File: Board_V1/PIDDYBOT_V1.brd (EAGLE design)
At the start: 48 x 76 mm, 76 parts, among them IC1 FT232RLSSOP, IC2 LMV358, IC3 LM1117, Q1 MOSFET-PCHANNELSMD, Q2 MOSFET-NCHANNELSMD, Q3 MOSFET-NCHANNELSMD, U1 MPU-6050-1, U2 MIC5205, U3 ATMEGA328, U4 TB6621FNG, U5 BLUETOOTH-RN41, Y1 16MHz

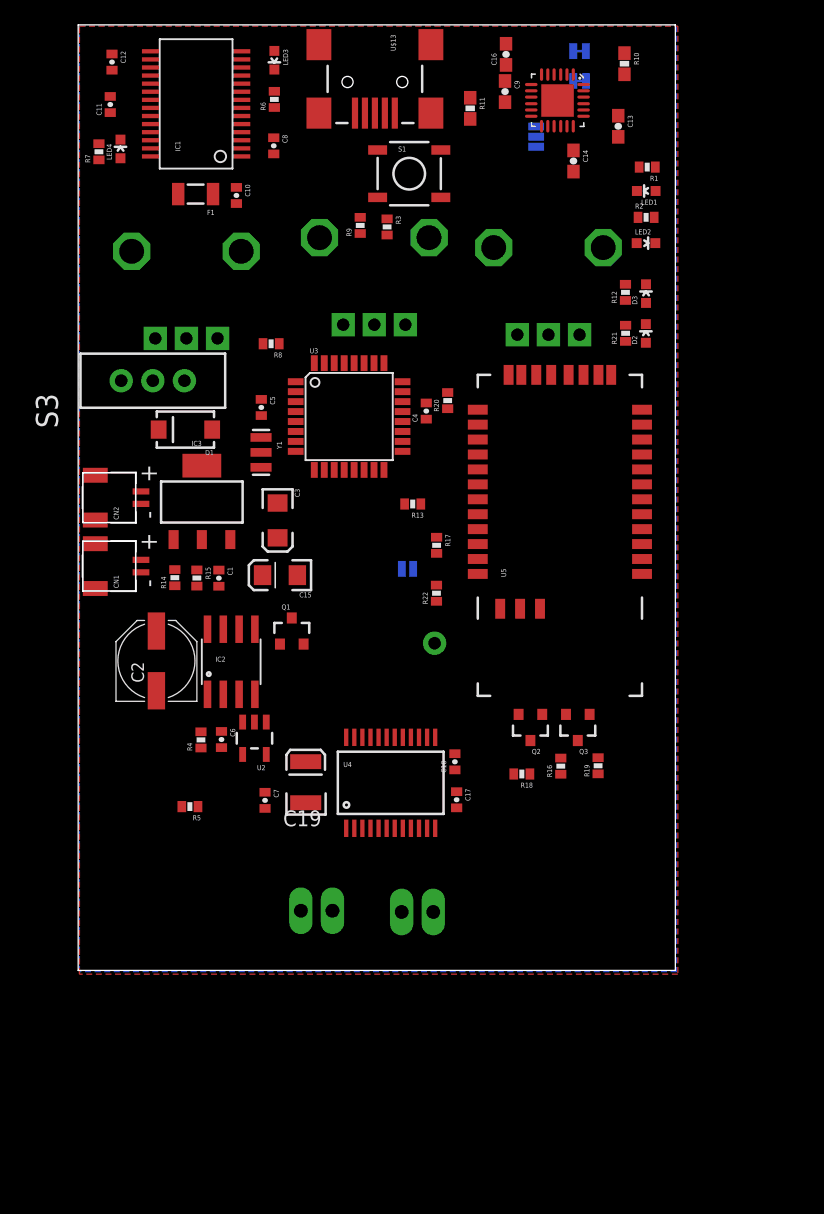
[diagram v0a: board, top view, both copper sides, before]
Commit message: Lots of Updates
Created second Simple Piddy.
Updates to Complex Piddy
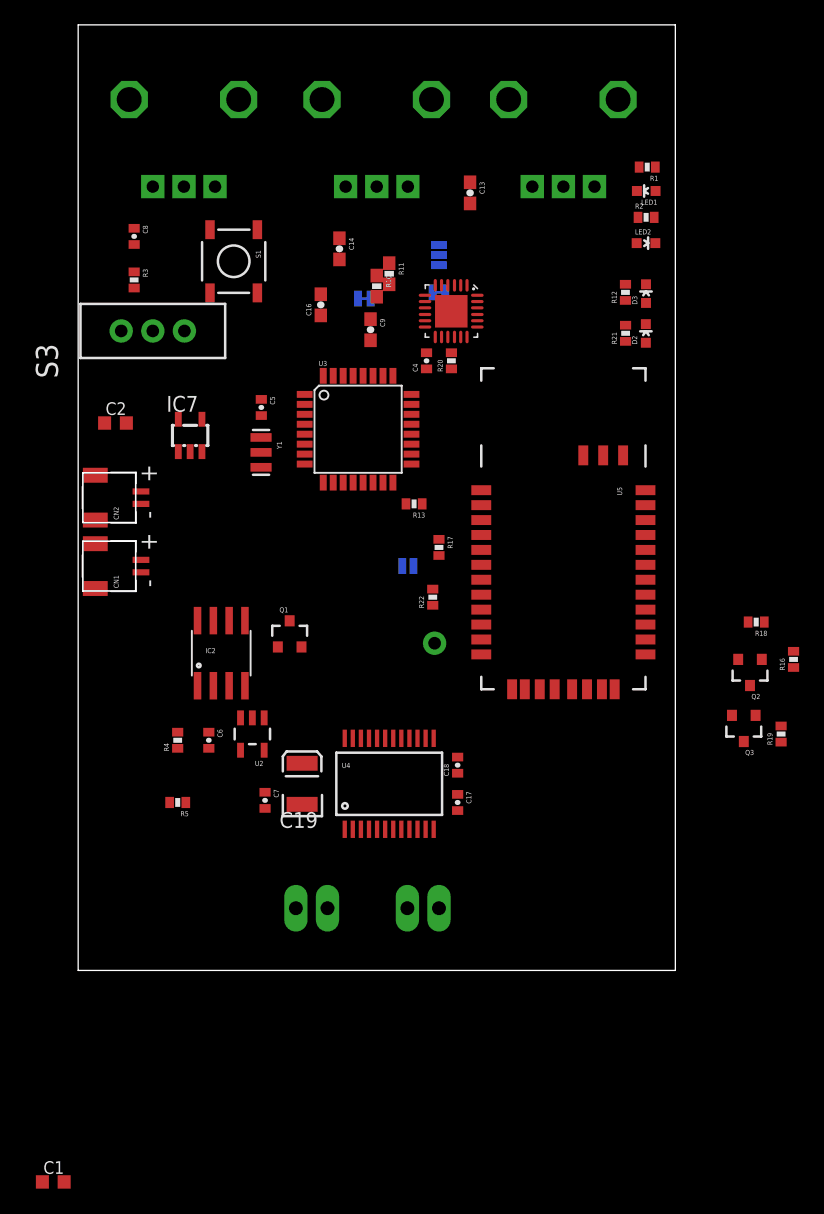
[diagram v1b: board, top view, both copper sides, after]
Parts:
- removed C10, C12: 0.1uF, SparkFun:0402-CAP
- removed C11: 0.1uF, SparkFun-Capacitors:0402-CAP
- removed C15: 10uF, SparkFun-Capacitors:EIA3216
- removed C3: 10uF, SparkFun:EIA3216
- removed D1: MBRA140, SparkFun:SMA-DIODE
- removed F1: 500mA, SparkFun:PTC-1206
- removed IC1: FT232RLSSOP, SparkFun-DigitalIC:SSOP28DB
- removed IC3: LM1117, Testing:SOT223-ALT1
- removed LED3: RED, SparkFun:LED-0603
- removed LED4: YELLOW, SparkFun:LED-0603
- removed R14: 715, SparkFun:0402-RES
- removed R15: 240, SparkFun:0402-RES
- removed R6, R7, R8, R9: 1k, SparkFun:0402-RES
- removed U$13: USB-MINIB-5PIN, SparkFun-Connectors:USB-MINIB
- added IC7: TLV71333DBV, anoven:SOT-23-5
- C1: value 0.1uF -> 100nF; device SparkFun:0402-CAP -> rcl:C0603K
- C2: value 47uF -> 100nF; device SparkFun:PANASONIC_D -> rcl:C0603K
- moved C1 50.3 mm to (-2.00, -17.0), turned to 0 degrees
- moved R10 26.8 mm to (24.0, 55.0)
- moved C16 25.0 mm to (19.5, 53.5)
- moved SJ3 24.6 mm to (23.0, 54.0)
- moved R18 22.5 mm to (54.5, 28.0)
- moved SJ2 22.4 mm to (29.0, 54.5)
- moved C9 22.0 mm to (23.5, 51.5)
- moved R3 20.8 mm to (4.50, 55.5)
- moved R16 20.6 mm to (57.5, 25.0)
- moved C14 20.1 mm to (21.0, 58.0)
- moved C2 19.4 mm to (3.00, 44.0), turned to 0 degrees
- moved U1 19.0 mm to (30.0, 53.0)
- moved Q2 18.2 mm to (54.0, 24.0)
- moved S1 15.8 mm to (12.5, 57.0), turned to 270 degrees
- moved R19 14.9 mm to (56.5, 19.0)
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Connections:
- removed net D+: IC1.15, U$13.D+
- removed net D-: IC1.16, U$13.D-
- removed net N$10: LED4.A, R7.2
- removed net N$12: CN1.2, CN2.1
- removed net N$13: CN2.2, S3.1
- removed net N$15: IC3.1, R14.2, R15.1
- removed net RXD: IC1.5, R9.2
- removed net RXLED: IC1.22, LED4.C
- removed net TXD: IC1.1, R8.2
- removed net TXLED: IC1.23, LED3.C
- removed net VIN1: C2.+, D1.C, IC3.3
- removed net VUSB: C10.1, F1.1, U$13.VBUS
- new net VBATT: C2.1, IC7.1, IC7.3
- new net VCC: C1.1, IC7.5
- new net V_BATT: S3.3
- net 5V: no longer C1.1, C11.1, C15.A, C3.A, IC1.20, IC1.4, IC3.2, IC3.4, R15.2, R6.1, R7.1
- net DTR: no longer IC1.2
- net GND: now also C2.2, CN2.1, IC7.2; no longer C10.2, C11.2, C12.2, C15.C, C2.-, C3.C, CN1.1, IC1.18, IC1.21, IC1.25, IC1.26, IC1.7, R14.1, U$13.GND, U$13.MTN1, U$13.MTN2, U$13.MTN3, U$13.MTN4
- net N$1: now also S3.2; no longer C12.1, IC1.17
- net N$8: now also CN1.1, CN2.2; no longer LED3.A, R6.2
- net PWRIN: no longer D1.A, S3.2
- net RX-I: no longer R8.1
- net TX-O: no longer R9.1
- net USBVCC: no longer F1.2
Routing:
- removed copper zone on layer 1, net GND
- removed copper zone on layer 16, net GND
